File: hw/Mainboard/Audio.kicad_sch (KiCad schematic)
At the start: 14 parts, among them J1 SJ-43504-SMT-TR, U22 LM386

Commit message: hw: wip
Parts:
- C30: LCSC C1525 -> C307331
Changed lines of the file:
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@@
       (effects (font (size 1.27 1.27)) hide)
     )
-    (property "Datasheet" "https://datasheet.lcsc.com/lcsc/1810191219_Samsung-Electro-Mechanics-CL05B104KO5NNNC_C1525.pdf" (id 3) (at 149.86 66.04 0)
+    (property "Datasheet" "" (id 3) (at 149.86 66.04 0)
       (effects (font (size 1.27 1.27)) hide)
     )
-    (property "LCSC" "C1525" (id 4) (at 149.86 66.04 0)
+    (property "LCSC" "C307331" (id 4) (at 149.86 66.04 0)
       (effects (font (size 1.27 1.27)) hide)
     )

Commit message: hw: wip
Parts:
- U22: MOUSER (none) -> 926-LM386N-1/NOPB
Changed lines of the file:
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@@
+      (effects (font (size 1.27 1.27)) hide)
+    )
+    (property "MOUSER" "926-LM386N-1/NOPB" (id 4) (at 167.64 73.66 0)
       (effects (font (size 1.27 1.27)) hide)
     )

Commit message: hw: wip
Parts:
- C55: footprint Capacitor_SMD:C_0402_1005Metric -> Capacitor_SMD:C_0603_1608Metric; LCSC C25118 -> C1622
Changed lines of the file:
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@@
       (effects (font (size 1.27 1.27)) hide)
     )
-    (property "Datasheet" "" (id 3) (at 149.86 66.04 0)
+    (property "Datasheet" "https://datasheet.lcsc.com/lcsc/2304140030_Samsung-Electro-Mechanics-CL05B104KB54PNC_C307331.pdf" (id 3) (at 149.86 66.04 0)
       (effects (font (size 1.27 1.27)) hide)
     )
@@
       (effects (font (size 1.27 1.27)) hide)
     )
-    (property "Datasheet" "~" (id 3) (at 87.63 96.52 0)
+    (property "Datasheet" "" (id 3) (at 87.63 96.52 0)
       (effects (font (size 1.27 1.27)) hide)
     )
@@
       (effects (font (size 1.27 1.27)) hide)
     )
-    (property "Datasheet" "~" (id 3) (at 87.63 88.9 0)
+    (property "Datasheet" "https://datasheet.lcsc.com/lcsc/2304140030_FH--Guangdong-Fenghua-Advanced-Tech-0402B223K500NT_C1532.pdf" (id 3) (at 87.63 88.9 0)
       (effects (font (size 1.27 1.27)) hide)
     )
@@
       (effects (font (size 1.27 1.27)) (justify left bottom) hide)
     )
-    (property "Datasheet" "https://www.mouser.com/datasheet/2/670/sj_43504_smt_tr-1779335.pdf" (id 3) (at 118.11 85.09 0)
+    (property "Datasheet" "" (id 3) (at 118.11 85.09 0)
       (effects (font (size 1.27 1.27)) (justify left bottom) hide)
     )
@@
       (effects (font (size 1.27 1.27)) hide)
     )
-    (property "Datasheet" "~" (id 3) (at 149.86 85.09 0)
+    (property "Datasheet" "" (id 3) (at 149.86 85.09 0)
       (effects (font (size 1.27 1.27)) hide)
     )
@@
       (effects (font (size 1.27 1.27)) hide)
     )
-    (property "Datasheet" "https://www.mouser.com/datasheet/2/334/AT-1220-TT-9-R-532252.pdf" (id 3) (at 209.296 74.93 0)
+    (property "Datasheet" "" (id 3) (at 209.296 74.93 0)
       (effects (font (size 1.27 1.27)) hide)
     )
@@
       (effects (font (size 1.27 1.27)) hide)
     )
-    (property "Datasheet" "~" (id 3) (at 157.48 62.23 0)
+    (property "Datasheet" "" (id 3) (at 157.48 62.23 0)
       (effects (font (size 1.27 1.27)) hide)
     )
@@
       (effects (font (size 1.27 1.27)) hide)
     )
-    (property "Datasheet" "http://www.ti.com/lit/ds/symlink/lm386.pdf" (id 3) (at 172.72 68.58 0)
+    (property "Datasheet" "" (id 3) (at 172.72 68.58 0)
       (effects (font (size 1.27 1.27)) hide)
     )
@@
       (effects (font (size 1.27 1.27)) hide)
     )
-    (property "Datasheet" "https://datasheet.lcsc.com/lcsc/1811091611_Samsung-Electro-Mechanics-CL05A105KA5NQNC_C52923.pdf" (id 3) (at 69.85 85.09 0)
+    (property "Datasheet" "https://datasheet.lcsc.com/lcsc/2304140030_Samsung-Electro-Mechanics-CL05A105KA5NQNC_C52923.pdf" (id 3) (at 69.85 85.09 0)
       (effects (font (size 1.27 1.27)) hide)
     )
@@
       (effects (font (size 1.27 1.27)) (justify left))
     )
-    (property "Footprint" "Capacitor_SMD:C_0402_1005Metric" (id 2) (at 181.61 80.01 0)
-      (effects (font (size 1.27 1.27)) hide)
-    )
-    (property "Datasheet" "~" (id 3) (at 181.61 80.01 0)
-      (effects (font (size 1.27 1.27)) hide)
-    )
-    (property "LCSC" "C25118" (id 4) (at 181.61 80.01 0)
+    (property "Footprint" "Capacitor_SMD:C_0603_1608Metric" (id 2) (at 181.61 80.01 0)
+      (effects (font (size 1.27 1.27)) hide)
+    )
+    (property "Datasheet" "https://datasheet.lcsc.com/lcsc/2304140030_Samsung-Electro-Mechanics-CL10B473KB8NNNC_C1622.pdf" (id 3) (at 181.61 80.01 0)
+      (effects (font (size 1.27 1.27)) hide)
+    )
+    (property "LCSC" "C1622" (id 4) (at 181.61 80.01 0)
       (effects (font (size 1.27 1.27)) hide)
     )
@@
       (effects (font (size 1.27 1.27)) hide)
     )
-    (property "Datasheet" "https://datasheet.lcsc.com/lcsc/1810221121_Samsung-Electro-Mechanics-CL31A476MPHNNNE_C96123.pdf" (id 3) (at 194.31 73.66 0)
-      (effects (font (size 1.27 1.27)) hide)
-    )
+    (property "Datasheet" "" (id 3) (at 194.31 73.66 0)
+      (effects (font (size 1.27 1.27)) hide)
+    )

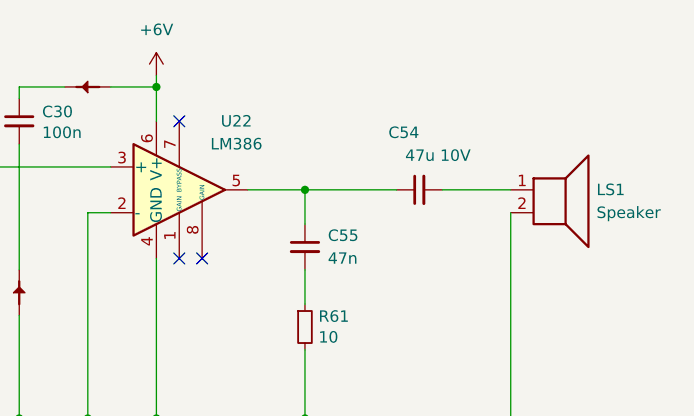
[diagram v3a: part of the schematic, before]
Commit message: wip
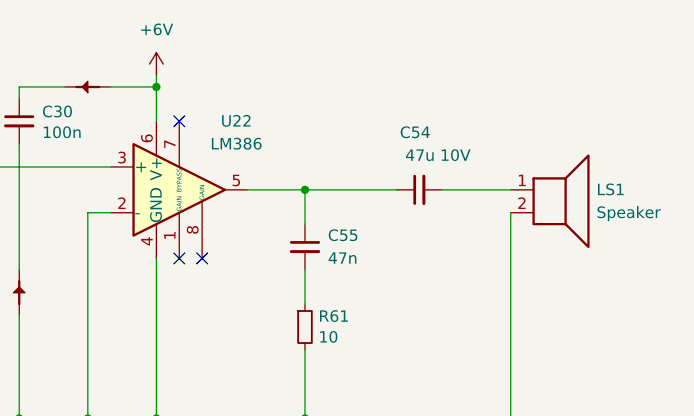
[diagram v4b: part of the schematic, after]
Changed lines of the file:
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@@
       (effects (font (size 1.27 1.27)) (justify left bottom) hide)
     )
-    (property "Datasheet" "" (id 3) (at 118.11 85.09 0)
+    (property "Datasheet" "https://www.mouser.com/datasheet/2/670/sj_43504_smt_tr-1779335.pdf" (id 3) (at 118.11 85.09 0)
       (effects (font (size 1.27 1.27)) (justify left bottom) hide)
     )
@@
   (symbol (lib_id "Device:C_Small") (at 194.31 73.66 90) (unit 1)
     (in_bom yes) (on_board yes)
-    (property "Reference" "C54" (id 0) (at 194.31 67.31 90)
+    (property "Reference" "C54" (id 0) (at 195.58 67.31 90)
       (effects (font (size 1.27 1.27)) (justify left))
     )
@@
       (effects (font (size 1.27 1.27)) hide)
     )
-    (property "Datasheet" "" (id 3) (at 194.31 73.66 0)
+    (property "Datasheet" "https://datasheet.lcsc.com/lcsc/2304140030_Samsung-Electro-Mechanics-CL31A476MPHNNNE_C96123.pdf" (id 3) (at 194.31 73.66 0)
       (effects (font (size 1.27 1.27)) hide)
     )
